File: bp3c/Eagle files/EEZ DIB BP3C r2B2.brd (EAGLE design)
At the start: 110 x 85 mm, 40 parts, among them IC1 PCA9536D, Q1 IRLML6244TRPBF, Q2 IRLML6244TRPBF, X1 ZL202-20G, X2 ZL202-20G, X3 ZL202-20G, X4 ZL212-40KG, X5 TSW-113-07-F-D, X6 TSW-113-07-F-D, X7 TSW-113-07-F-D

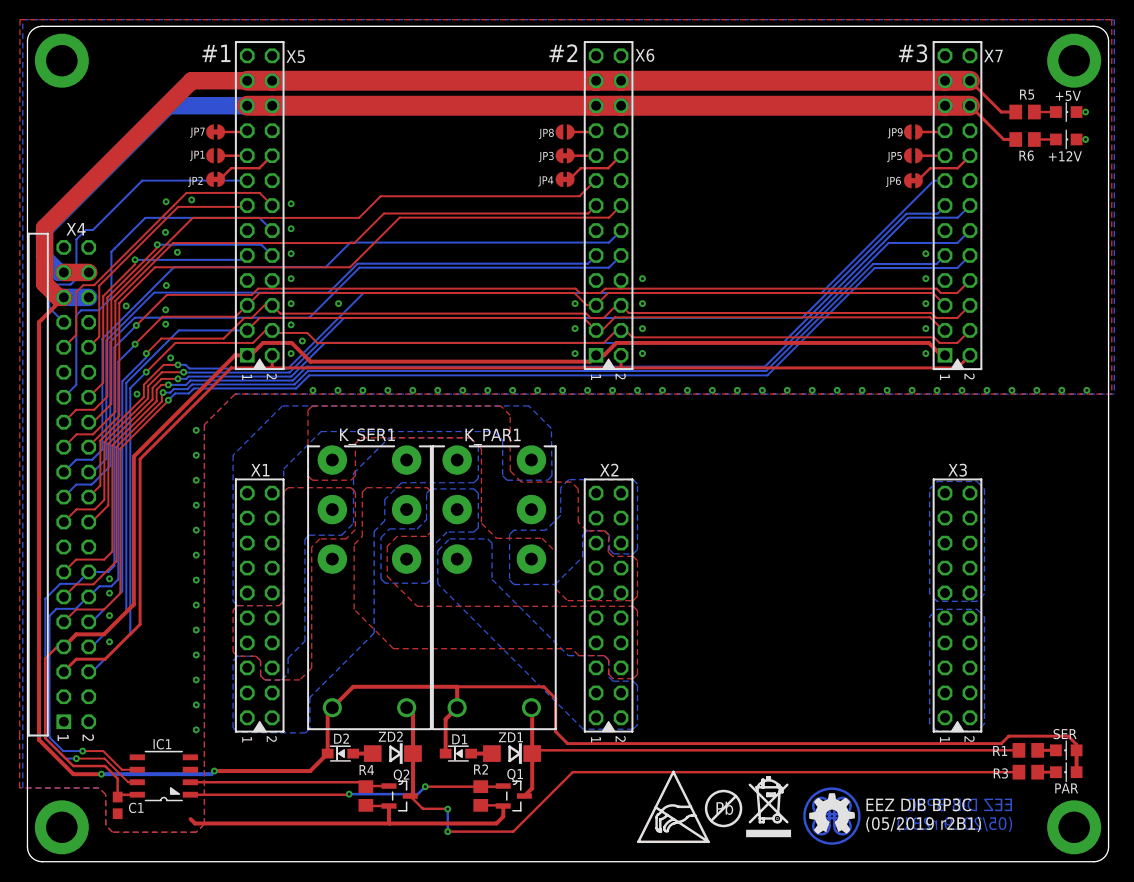
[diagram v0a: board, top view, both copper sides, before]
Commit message: #38
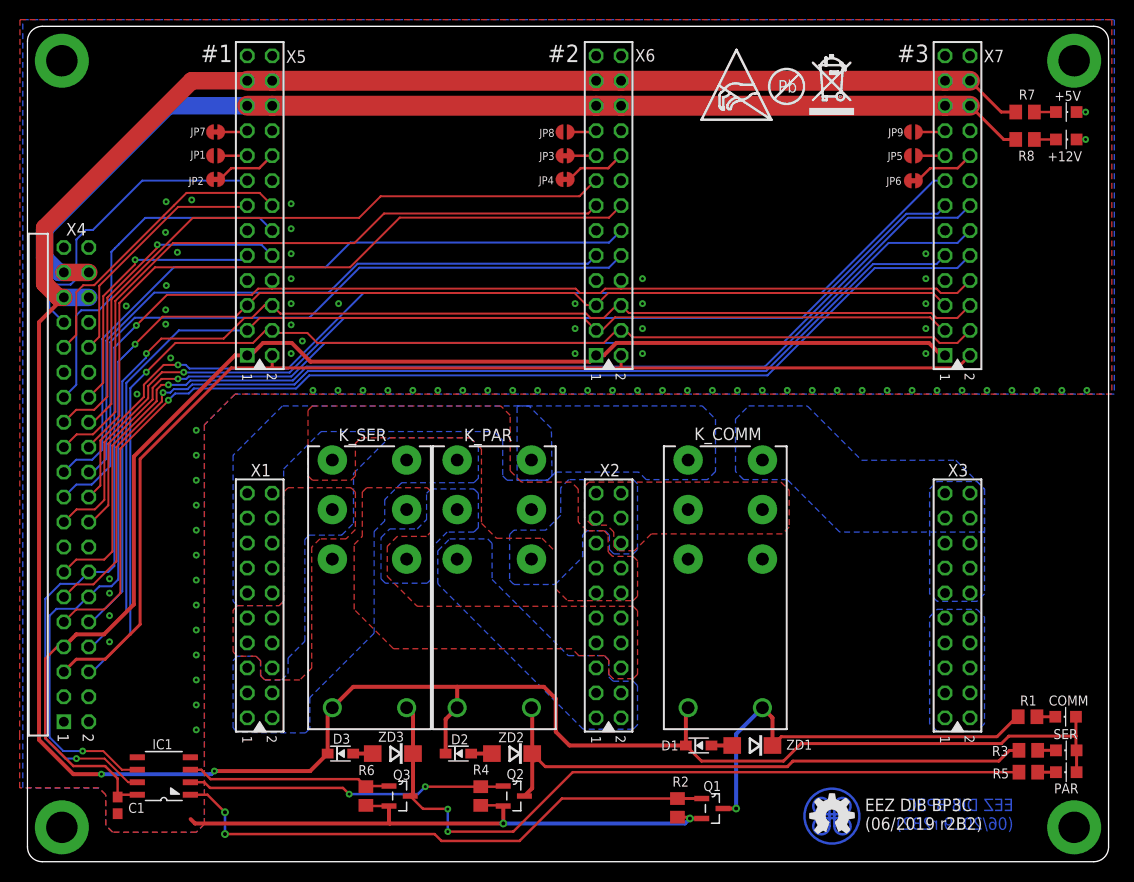
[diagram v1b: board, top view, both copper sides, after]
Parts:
- added COMM: Green, EEZ_Lib1:LED_0805
- added D3: BAS316, EEZ_Lib1:SOD323-R
- added K_COMM: RT424005, EEZ_Lib1:RT-C/016A5_ROUND
- added Q3: IRLML6244TRPBF, EEZ_Lib1:SOT103P240X110-3N
- added R7: 470R, rcl:R0805
- added R8: 1K5, rcl:R0805
- added ZD3: SMAJ18A, EEZ_Lib1:DO214AC
- R5: value 470R -> 330R
- R6: value 1K5 -> 100K
- moved R6 94.7 mm to (24.4, 11.7), turned to 90 degrees
- moved U$2 73.7 mm to (69.5, 81.0)
- moved U$4 73.7 mm to (58.6, 80.5)
- moved U$5 73.7 mm to (67.2, 83.9)
- moved R5 67.2 mm to (91.8, 14.1), turned to 180 degrees
- moved D1 24.5 mm to (58.3, 16.8)
- moved ZD1 24.5 mm to (63.8, 16.8)
- moved Q1 20.2 mm to (59.7, 10.4)
- moved R2 20.1 mm to (56.1, 10.5)
- moved ZD2 12.1 mm to (39.3, 16.0)
- moved D2 12.0 mm to (33.8, 16.0)
- moved R4 11.7 mm to (36.1, 11.7)
- moved Q2 11.6 mm to (39.5, 11.7)
- moved R1 3.42 mm to (91.8, 19.7)
- moved R3 2.22 mm to (91.8, 16.3)
- renumbered K_PAR1 to K_PAR, K_SER1 to K_SER
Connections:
- new net N$104: D3.A, ZD3.A
- new net N$17: K_COMM.A1, Q1.3, R1.2, ZD1.C
- new net N$19: COMM.C, R1.1
- new net OUT_PAR1: IC1.1, Q1.1, R2.2
- net +12V: now also R8.1; no longer R6.1
- net +5V: now also COMM.A, D3.C, K_COMM.A2, R7.1; no longer R5.1
- net CH1_OUT-: now also K_COMM.14A
- net CH2_OUT-: now also K_COMM.11A, K_COMM.11B
- net CH3-: now also K_COMM.14B
- net GND: now also Q3.2, R6.1
- net N$101: now also Q3.3, R5.2, ZD3.C; no longer Q2.3, R3.2, ZD2.C
- net N$102: now also Q2.3, R3.2, ZD2.C; no longer Q1.3, R1.2, ZD1.C
- net N$3: now also R7.2; no longer R5.2
- net N$4: now also R8.2; no longer R6.2
- net N$7: now also R5.1; no longer R3.1
- net N$8: now also R3.1; no longer R1.1
- net OUT_PAR: now also IC1.2, Q2.1, R4.2; no longer IC1.1, Q1.1, R2.2
- net OUT_SER: now also IC1.3, Q3.1, R6.2; no longer IC1.2, Q2.1, R4.2
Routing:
- net OUT_PAR1: track 0.00 -> 57.1 mm, vias 0 -> 2
- net N$17: track 0.00 -> 43.2 mm, vias 0 -> 1
- net GND: track 39.9 -> 62.0 mm, vias 82 -> 84
- net +5V: track 291.4 -> 299.4 mm
- net N$102: track 59.0 -> 62.0 mm
- net N$104: track 0.00 -> 1.98 mm
- net N$19: track 0.00 -> 1.87 mm
- net OUT_SER: track 20.4 -> 21.6 mm
- net OUT_PAR: track 32.2 -> 32.8 mm
- added copper zone on layer 1, net CH2_OUT-
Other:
- board text added: "EEZ DIB BP3C (06/2019 r2B2)"
- board text removed: "EEZ DIB BP3C (05/2019 r2B1)"

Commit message: #39
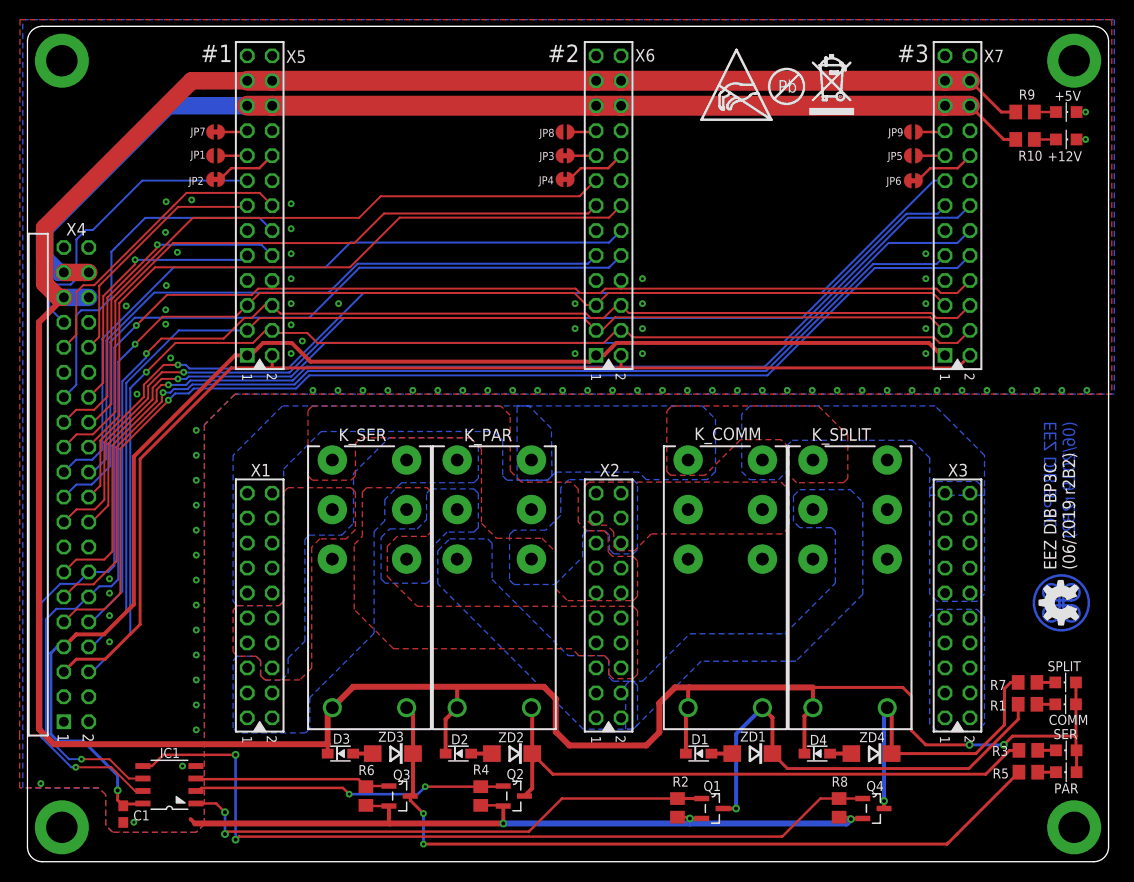
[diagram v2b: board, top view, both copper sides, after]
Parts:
- added D4: BAS316, EEZ_Lib1:SOD323-R
- added K_SPLIT: RT424005, EEZ_Lib1:RT-C/016A5_ROUND
- added Q4: IRLML6244TRPBF, EEZ_Lib1:SOT103P240X110-3N
- added R10: 1K5, rcl:R0805
- added R9: 470R, rcl:R0805
- added SPLIT: Green, EEZ_Lib1:LED_0805
- added ZD4: SMAJ18A, EEZ_Lib1:DO214AC
- R7: value 470R -> 330R
- R8: value 1K5 -> 100K
- moved R8 70.6 mm to (72.6, 10.5), turned to 90 degrees
- moved R7 58.0 mm to (91.8, 23.2), turned to 180 degrees
- moved EEZ_SIGNATURE 31.9 mm to (95.2, 31.3), turned to 270 degrees
- moved COMM 1.27 mm to (95.6, 21.0)
- moved R1 1.27 mm to (91.8, 21.0)
- moved C1 1.06 mm to (-0.25, 9.84)
- moved IC1 1.06 mm to (4.45, 12.8)
- moved D1 0.83 mm to (58.3, 16.0)
- moved ZD1 0.83 mm to (63.8, 16.0)
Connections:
- net OUT_PAR1 renamed OUT_COMM
- new net N$20: K_SPLIT.A1, Q4.3, R7.2, ZD4.C
- new net N$21: D4.A, ZD4.A
- new net N$22: R7.1, SPLIT.C
- new net OUT_SPLIT: IC1.5, Q4.1, R8.2
- net +12V: now also R10.1; no longer R8.1
- net +5V: now also D4.C, K_SPLIT.A2, R9.1, SPLIT.A; no longer R7.1
- net CH1_OUT-: now also K_SPLIT.14A
- net CH2_OUT+: now also K_SPLIT.11A
- net GND: now also Q4.2, R8.1
- net N$3: now also R9.2; no longer R7.2
- net N$4: now also R10.2; no longer R8.2
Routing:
- net OUT_SPLIT: track 0.00 -> 84.1 mm, vias 0 -> 2
- net N$20: track 0.00 -> 33.3 mm, vias 0 -> 1
- net GND: track 62.0 -> 81.4 mm, vias 84 -> 88
- net +5V: track 299.4 -> 317.4 mm
- net N$17: track 43.2 -> 47.0 mm
- net N$21: track 0.00 -> 2.17 mm
- net N$22: track 0.00 -> 1.87 mm
- net N$101: track 76.7 -> 78.4 mm
- net OUT_COMM: track 57.1 -> 55.6 mm
- net I2C1_SCL: track 142.0 -> 143.4 mm
- net I2C1_SDA: track 148.4 -> 149.8 mm
- net N$102: track 62.0 -> 62.7 mm
- net +3V3: track 136.9 -> 137.2 mm, vias 0 -> 1
- added copper zone on layer 1, net CH1_OUT-
